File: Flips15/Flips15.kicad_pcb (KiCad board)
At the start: 2 copper layers, 100 x 100 mm, 68 parts, among them CN1 UFP2810, U1001 74HC238, U1002 ULN2803A, U1003 74HC238, U1004 TBD62783A, U1101 74HC238, U1102 ULN2803A, U1103 74HC238, U1104 TBD62783A, U701 74HC238, U801 74HC238, U802 ULN2803A, U803 74HC238, U804 TBD62783A, U901 74HC238, U902 ULN2803A, U903 74HC238, U904 TBD62783A

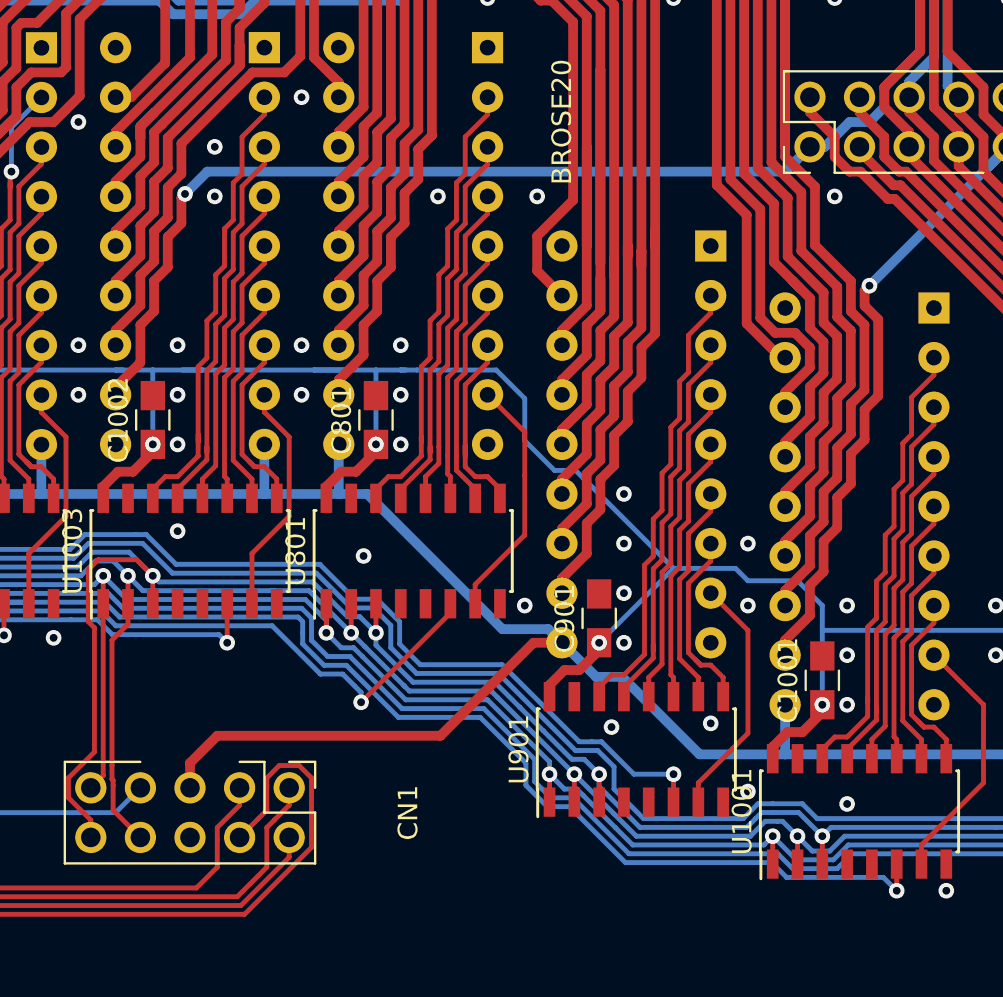
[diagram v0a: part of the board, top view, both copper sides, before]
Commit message: improve traces
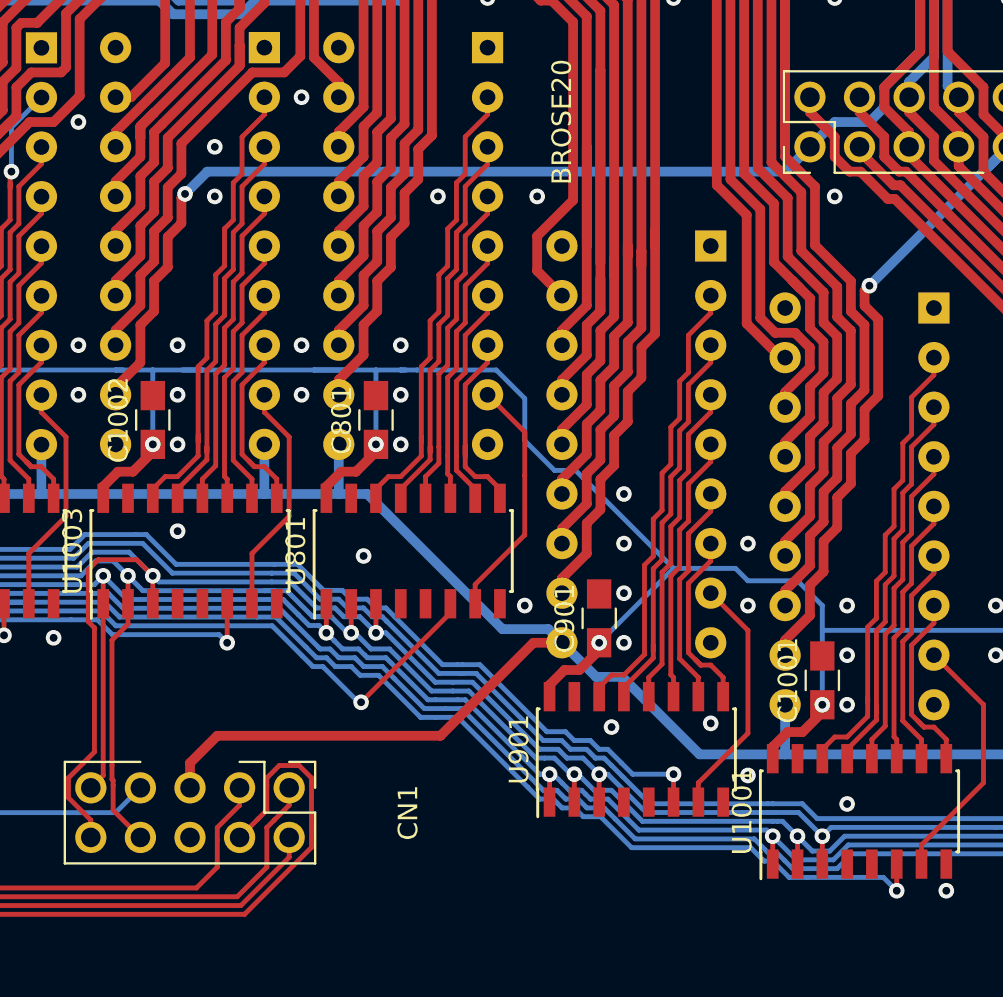
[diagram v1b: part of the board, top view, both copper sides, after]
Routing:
- net /UnitY/E3L: track 100.2 -> 98.2 mm
- net /UnitY/A2: track 123.7 -> 122.3 mm
- net /UnitY/E2L: track 70.5 -> 69.2 mm
- net /UnitY/E3H: track 90.2 -> 88.8 mm
- net /UnitY/A0: track 114.5 -> 113.4 mm
- net /UnitY/E1L: track 68.4 -> 67.8 mm
